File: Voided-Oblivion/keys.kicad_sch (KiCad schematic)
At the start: 170 parts, among them U8 SN74LVC2T45DCUR

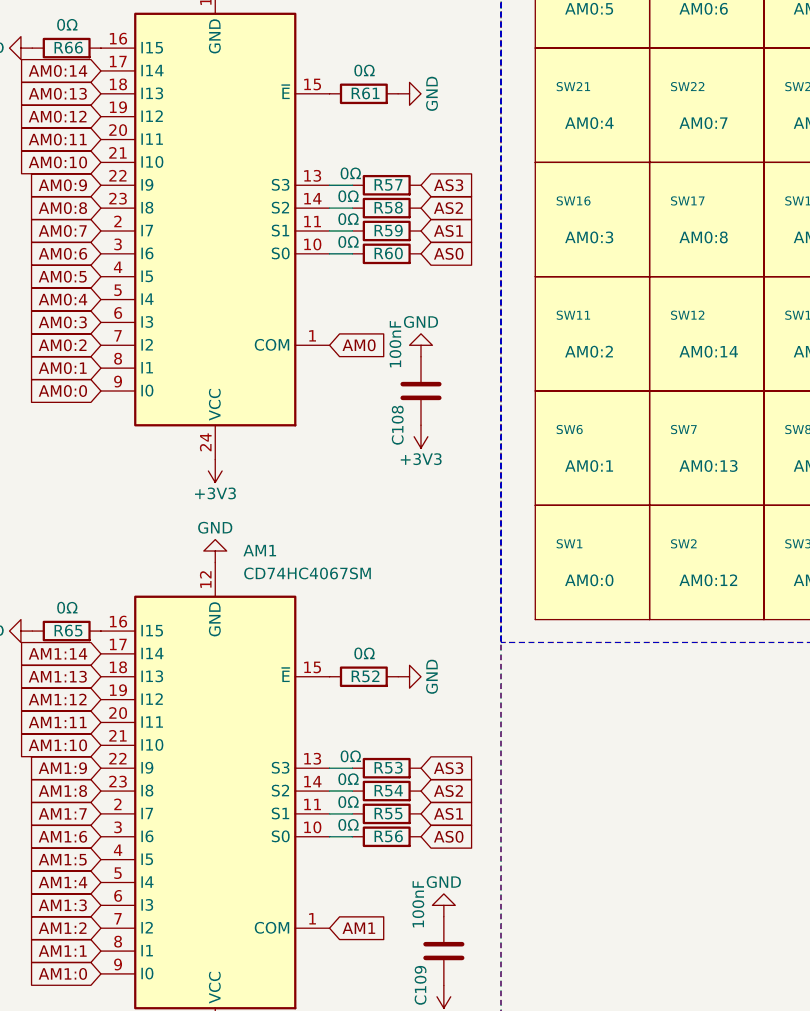
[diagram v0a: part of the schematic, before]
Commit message: still cis tho
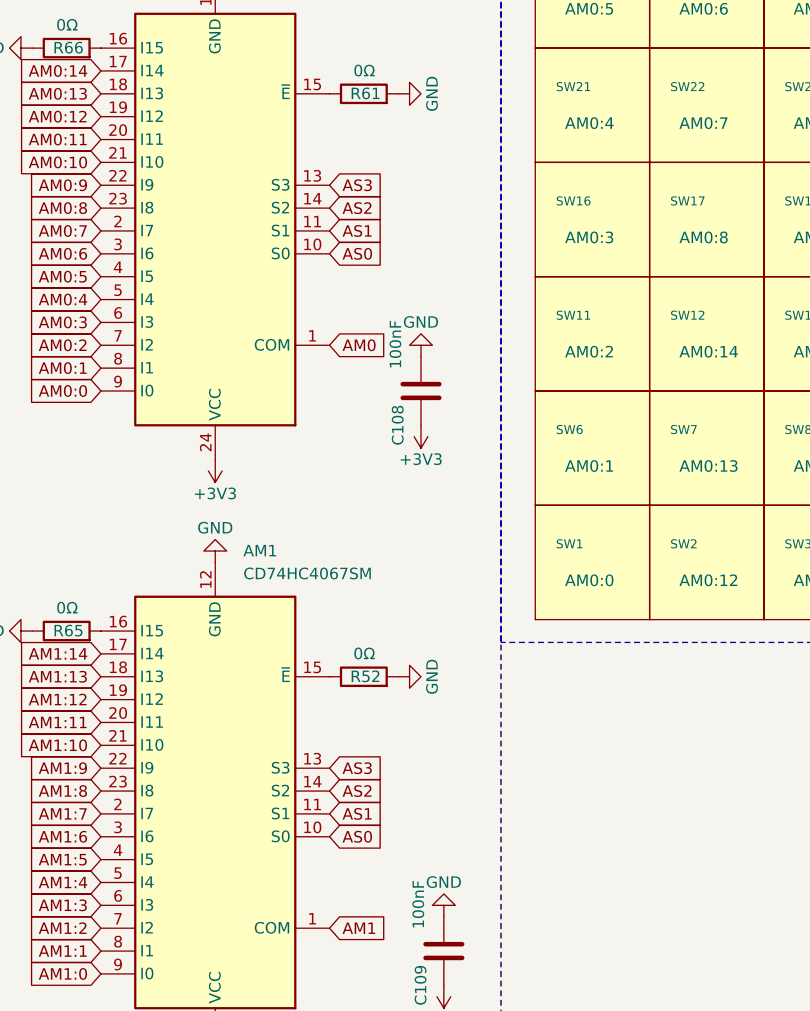
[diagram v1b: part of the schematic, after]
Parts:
- removed R53, R54, R55, R56, R57, R58, R59, R60: 0Ω, Resistor_SMD:R_0402_1005Metric, symbol Device:R
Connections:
- net AS0: now also AM0.10 (S0), AM1.10 (S0)
- net AS1: now also AM0.11 (S1), AM1.11 (S1)
- net AS2: now also AM0.14 (S2), AM1.14 (S2)
- net AS3: now also AM0.13 (S3), AM1.13 (S3)

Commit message: small changes
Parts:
- C100, C101, C102, C103, C104, C105, C106, C107, C108, C109, C46, C47, C48, C49, C50, C51, C52, C53, C54, C55, C56, C57, C58, C59, C60, C61, C62, C63, C64, C65, C66, C67, C68, C69, C70, C71, C72, C73, C74, C75, C78, C79, C80, C81, C82, C83, C84, C85, C86, C87, C88, C89, C90, C91, C92, C93, C94, C95, C96, C97, C98, C99: footprint Capacitor_SMD:C_0402_1005Metric -> Voided-Oblivion-misc:C_0402_1005Metric-no-silkscreen-text
- R52, R61, R62, R63, R64, R65, R66: footprint Resistor_SMD:R_0402_1005Metric -> Voided-Oblivion-misc:R_0402_1005Metric-no-silkscreen-text
